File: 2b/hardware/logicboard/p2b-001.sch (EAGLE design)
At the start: 76 parts, among them IC1 74LS06N, IC2 4066N, J1 MKR, J10 1-Wire, J2 GPIO, J20 GPIO, J3 Vcc, J4** RLY2, J5 SPI, J6 LED, J7 DIN5, J8 DIN5, J9 DIN5, K1 G5V1, Q1 220mA/50V/3.5Ω, Q2 220mA/50V/3.5Ω, T1 2SC1815

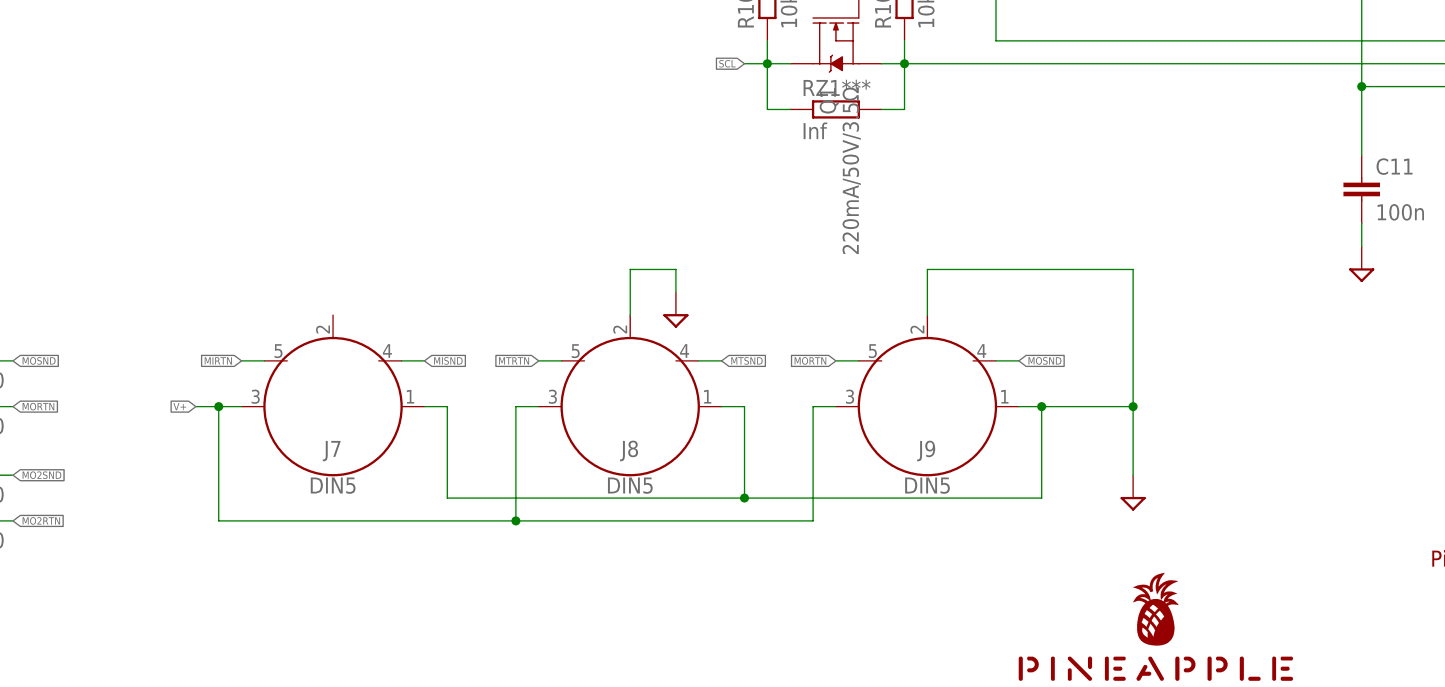
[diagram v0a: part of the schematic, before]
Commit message: Added SW.
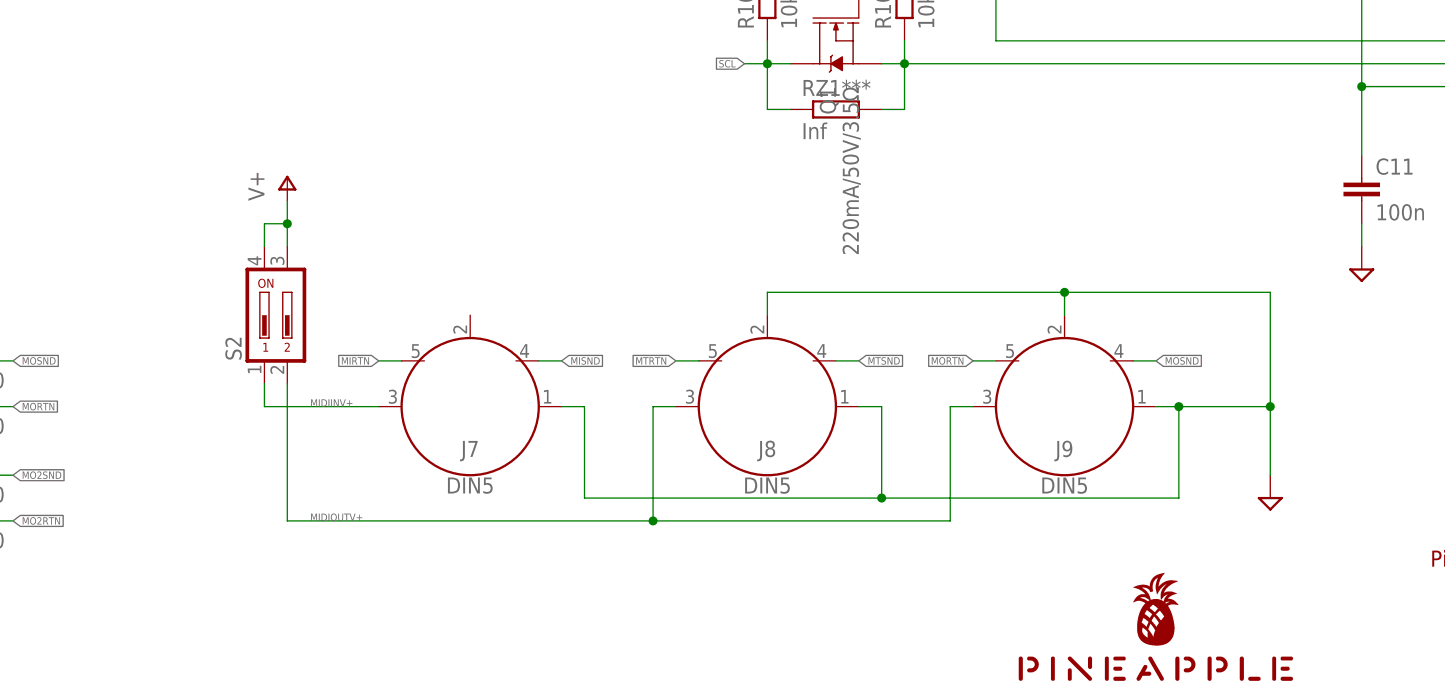
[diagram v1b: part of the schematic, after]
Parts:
- added S2: (no value), switch-dil:DIP02YL
- V1: device v-reg:78XXL -> v-reg:78XXS
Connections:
- new net MIDIINV+: J7.3, S2.1
- new net MIDIOUTV+: J8.3, J9.3, S2.2
- net V+: now also S2.3, S2.4; no longer J7.3, J8.3, J9.3
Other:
- moved on the sheet: J7, J8, J9

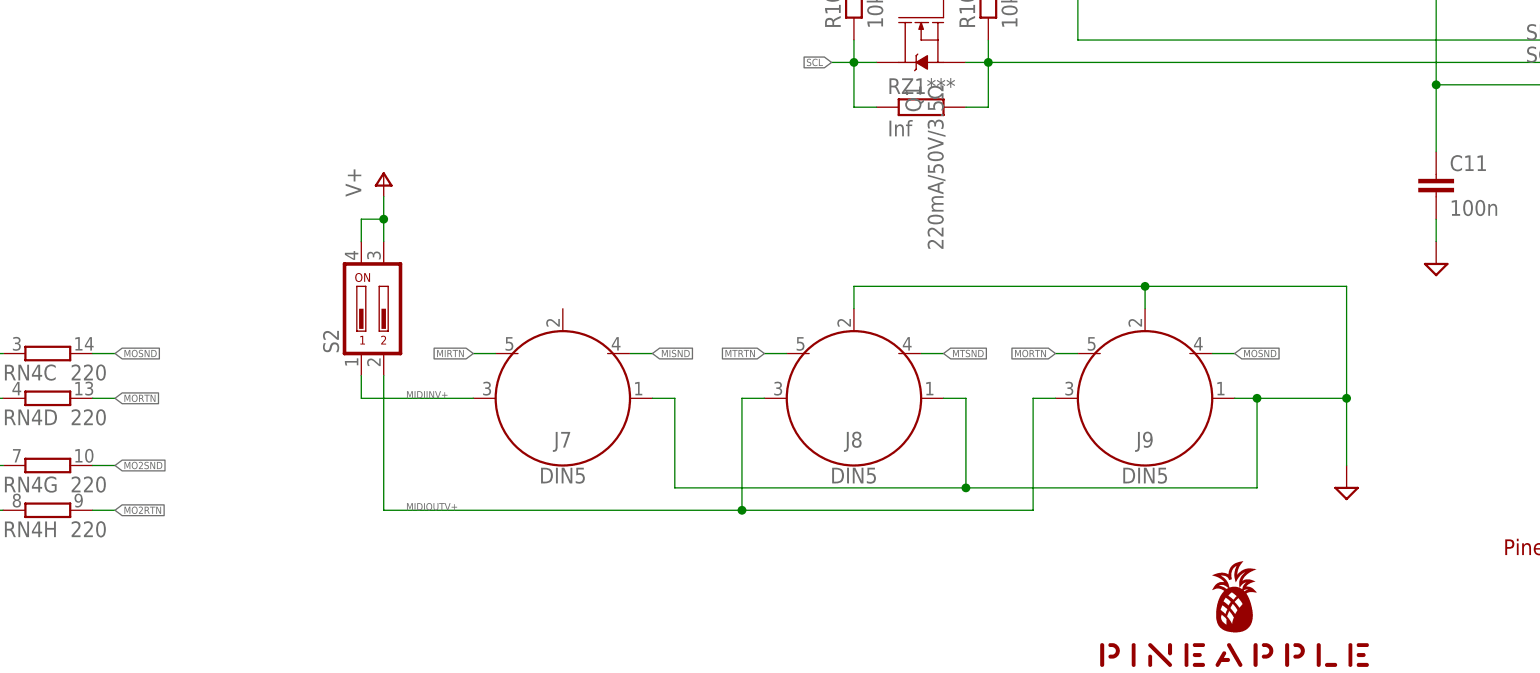
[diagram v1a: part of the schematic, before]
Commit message: Now has a phantom SW.
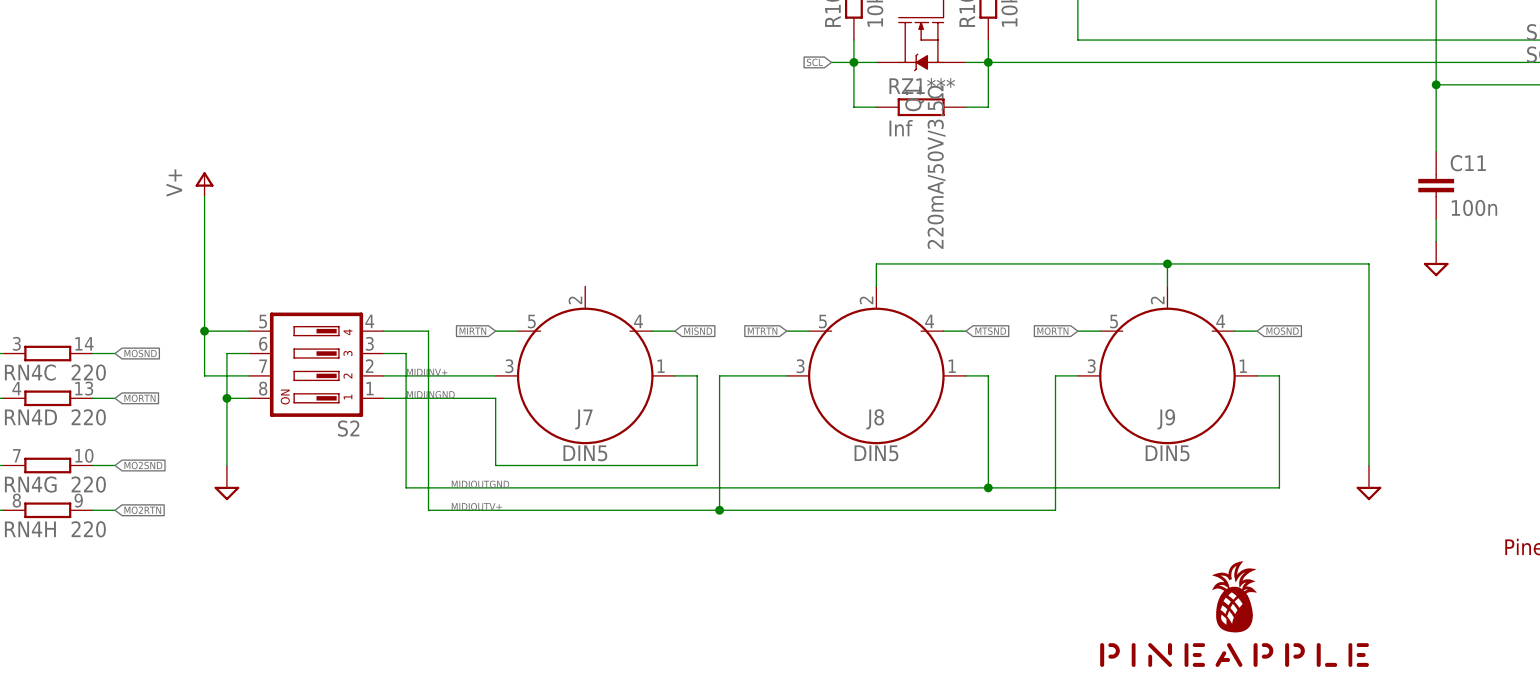
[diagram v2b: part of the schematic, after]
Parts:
- S2: device switch-dil:DIP02YL -> switch-dil:DIP04YL
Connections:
- new net MIDIINGND: J7.1, S2.1
- new net MIDIOUTGND: J8.1, J9.1, S2.3
- net GND: now also S2.6, S2.8; no longer J7.1, J8.1, J9.1
- net MIDIINV+: now also S2.2; no longer S2.1
- net MIDIOUTV+: now also S2.4; no longer S2.2
- net V+: now also S2.5, S2.7; no longer S2.3, S2.4
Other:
- moved on the sheet: J7, J8, J9
